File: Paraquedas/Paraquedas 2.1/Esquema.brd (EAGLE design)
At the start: 67.5 x 58.3 mm, 20 parts, among them Q1 IRF540, Q2 IRF540, Q3 IRF540

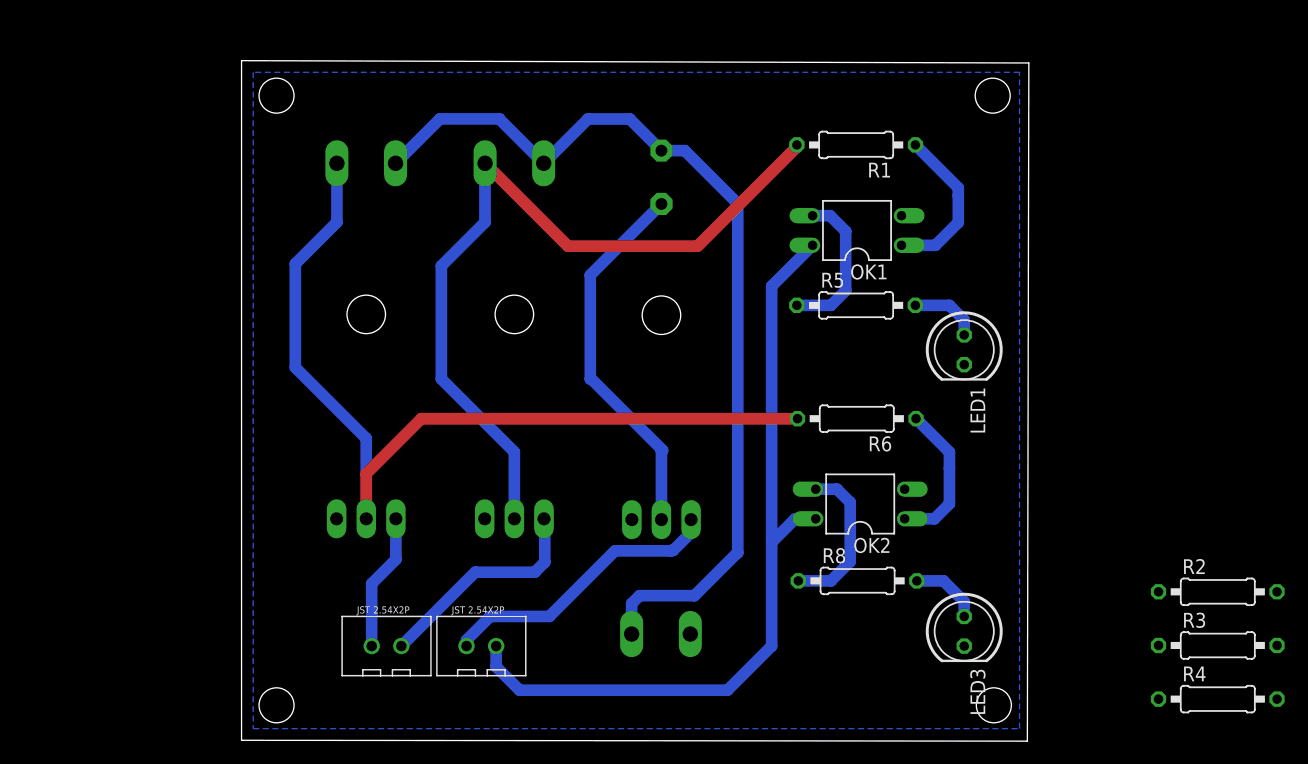
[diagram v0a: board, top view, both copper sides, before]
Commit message: Message
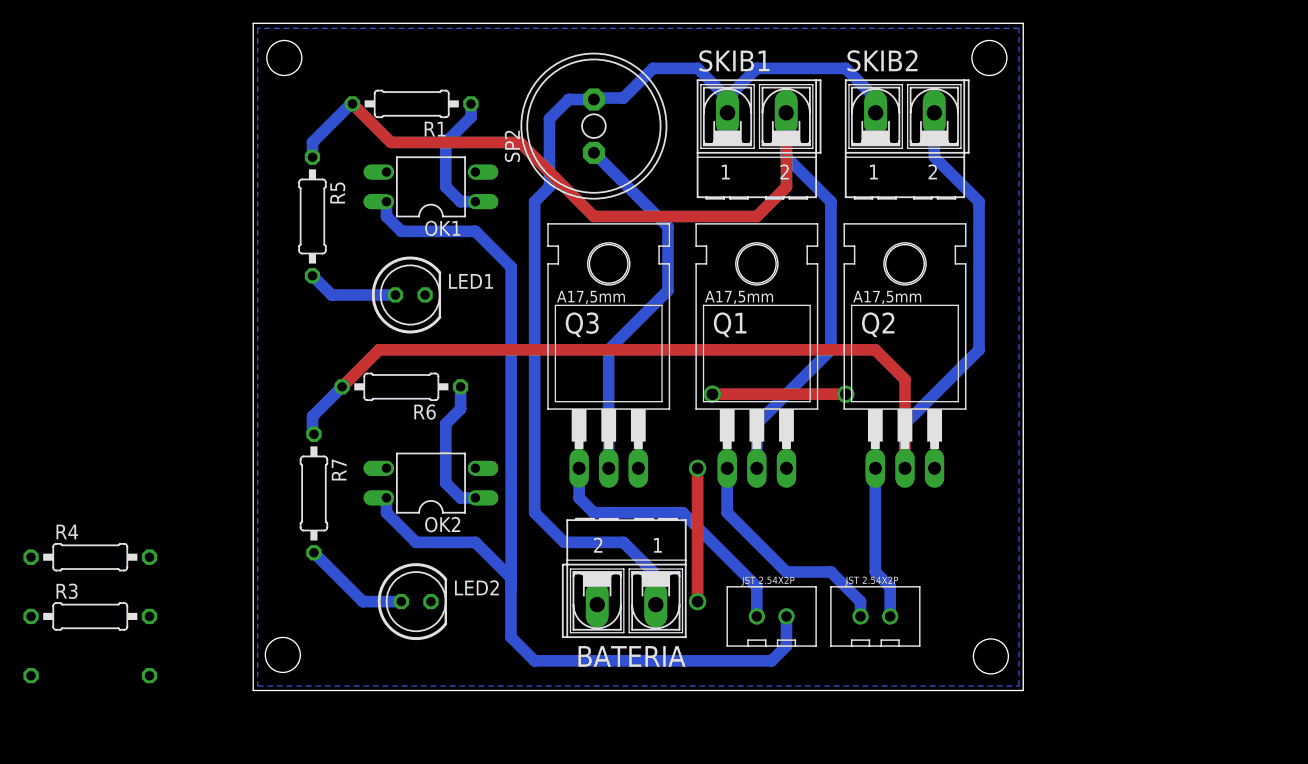
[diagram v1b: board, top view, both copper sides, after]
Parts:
- removed LED3: 5mm, led:LED5MM
- removed R8: 220, rcl:0207/10
- added LED2: 5mm, led:LED5MM
- added R7: 1k, rcl:0207/10
- R1, R5: value 220 -> 1k
- moved R4 97.4 mm to (-14.0, 11.4)
- moved R2 96.9 mm to (-14.0, 1.27), flipped to the bottom, turned to 180 degrees
- moved R3 96.7 mm to (-14.0, 6.35)
- moved LED1 47.7 mm to (13.5, 33.9), turned to 0 degrees
- moved R5 47.2 mm to (5.08, 40.6), turned to 270 degrees
- moved Q2 46.4 mm to (55.9, 25.4), flipped to the top
- moved SKIB2 46.4 mm to (55.9, 49.5), flipped to the top
- moved U$2 42.0 mm to (53.3, 6.35)
- moved R6 39.1 mm to (12.7, 26.0)
- moved R1 38.3 mm to (13.6, 50.3)
- moved OK2 36.8 mm to (15.2, 17.8)
- moved OK1 36.7 mm to (15.2, 43.2)
- moved U$1 25.0 mm to (44.5, 6.35)
- moved Q1 21.2 mm to (43.2, 25.4), flipped to the top
- moved SKIB1 21.2 mm to (43.2, 49.5), flipped to the top
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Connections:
- removed net N$3 (its old number): LED3.A, R8.2
- new net N$1: LED2.A, R7.2
- net GND: now also LED2.K; no longer LED3.K
- net SINAL_SKIB1: no longer R5.1
- net SINAL_SKIB2: no longer R8.1
- net SKIB1: now also U$2.1; no longer U$2.2
- net SKIB1_CONECTOR: now also R5.1
- net SKIB2: now also U$2.2; no longer U$2.1
- net SKIB2_CONECTOR: now also R7.1
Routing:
- net GND: track 0.00 -> 22.9 mm, vias 0 -> 4
- net SKIB1_CONECTOR: track 68.0 -> 89.4 mm
- net SKIB2_CONECTOR: track 77.3 -> 98.1 mm
- net 3.3V: track 68.2 -> 88.0 mm
- net SINAL_SKIB2: track 13.6 -> 0.00 mm
- net SINAL_SKIB1: track 13.2 -> 0.00 mm
- net N$1: track 0.00 -> 9.23 mm
- net N$3 (its old number): track 6.07 -> 0.00 mm
- net VCC: track 80.5 -> 86.2 mm
- net N$4: track 13.9 -> 11.1 mm
- net N$3: track 5.99 -> 7.80 mm
- net SKIB2: track 11.8 -> 13.2 mm
- net BUZZER: track 24.7 -> 23.5 mm
- net N$5: track 12.9 -> 11.8 mm
- net SKIB1: track 19.0 -> 19.7 mm
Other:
- board size 67.5 x 58.3 mm -> 66 x 57.2 mm
